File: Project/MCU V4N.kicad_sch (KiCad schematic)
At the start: 22 parts, among them J1 Conn_01x04, J10 Conn_01x01, J11 Conn_01x01, J2 Conn_01x01, J3 Conn_01x01, J4 Conn_01x01, J5 Conn_01x01, J6 Conn_01x01, J7 Conn_01x01, J8 Conn_01x01, J9 Conn_01x01, U53 STM32F072CBT6

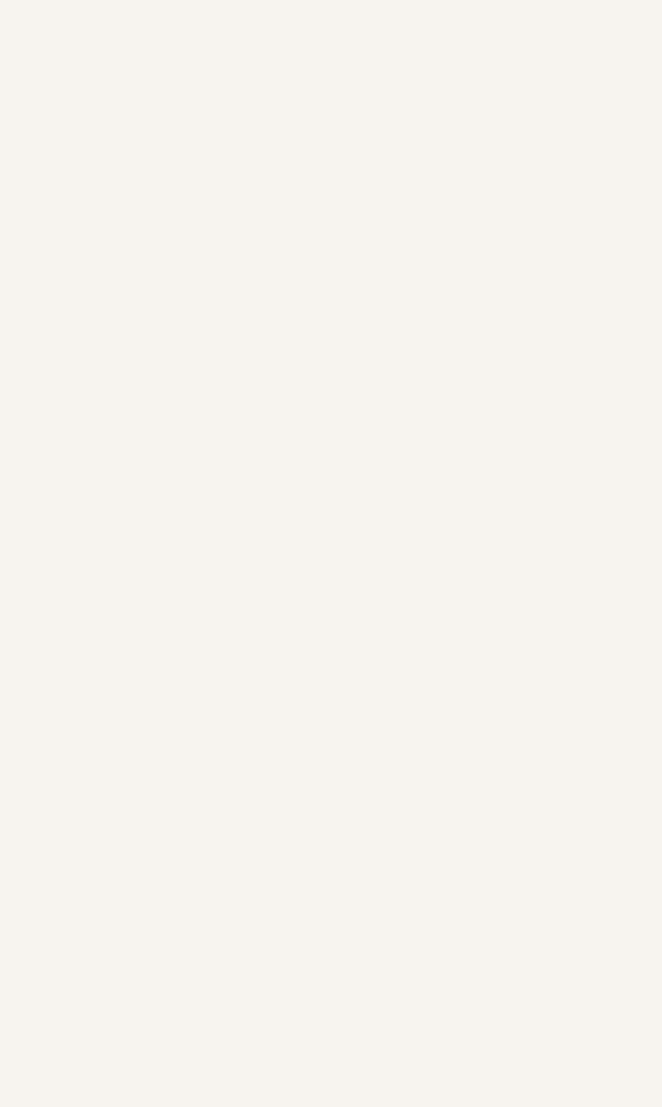
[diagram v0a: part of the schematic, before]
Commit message: revision work
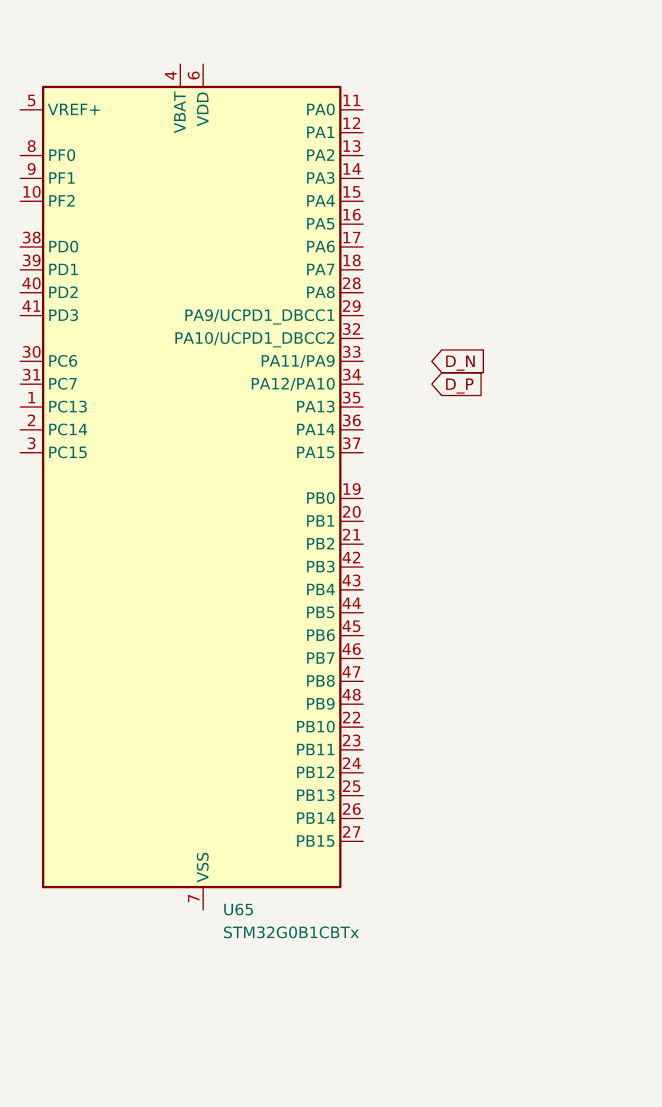
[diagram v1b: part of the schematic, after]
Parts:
- added U65: STM32G0B1CBTx, Package_QFP:LQFP-48_7x7mm_P0.5mm, symbol MCU_ST_STM32G0:STM32G0B1CBTx
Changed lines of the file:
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@@
+		)
+	)
+	(global_label "D_N"
+		(shape input)
+		(at -15.24 50.8 0)
+		(fields_autoplaced yes)
+		(effects
+			(font
+				(size 1.27 1.27)
+			)
+			(justify left)
+		)
+		(property "Intersheetrefs" "${INTERSHEET_REFS}"
+			(at -8.7661 50.8 0)
+			(effects
+				(font
+					(size 1.27 1.27)
+				)
+				(justify left)
+				(hide yes)
+			)
 		)
 	)
@@
 				)
 				(justify right)
+				(hide yes)
+			)
+		)
+	)
+	(global_label "D_P"
+		(shape input)
+		(at -15.24 53.34 0)
+		(fields_autoplaced yes)
+		(effects
+			(font
+				(size 1.27 1.27)
+			)
+			(justify left)
+		)
+		(property "Intersheetrefs" "${INTERSHEET_REFS}"
+			(at -8.8266 53.34 0)
+			(effects
+				(font
+					(size 1.27 1.27)
+				)
+				(justify left)
 				(hide yes)
 			)
@@
 					(unit 1)
 				)
+			)
+		)
+	)
+	(symbol
+		(lib_id "MCU_ST_STM32G0:STM32G0B1CBTx")
+		(at -43.18 66.04 0)
+		(unit 1)
+		(exclude_from_sim no)
+		(in_bom yes)
+		(on_board yes)
+		(dnp no)
+		(fields_autoplaced yes)
+		(property "Reference" "U65"
+			(at -38.4459 111.76 0)
+			(effects
+				(font
+					(size 1.27 1.27)
+				)
+				(justify left)
+			)
+		)
+		(property "Value" "STM32G0B1CBTx"
+			(at -38.4459 114.3 0)
+			(effects
+				(font
+					(size 1.27 1.27)
+				)
+				(justify left)
+			)
+		)
+		(property "Footprint" "Package_QFP:LQFP-48_7x7mm_P0.5mm"
+			(at -58.42 109.22 0)
+			(effects
+				(font
+					(size 1.27 1.27)
+				)
+				(justify right)
+				(hide yes)
+			)
+		)
+		(property "Datasheet" "https://www.st.com/resource/en/datasheet/stm32g0b1cb.pdf"
+			(at -43.18 66.04 0)
+			(effects
+				(font
+					(size 1.27 1.27)
+				)
+				(hide yes)
+			)
+		)
+		(property "Description" "STMicroelectronics Arm Cortex-M0+ MCU, 128KB flash, 144KB RAM, 64 MHz, 1.7-3.6V, 44 GPIO, LQFP48"
+			(at -43.18 66.04 0)
+			(effects
+				(font
+					(size 1.27 1.27)
+				)
+				(hide yes)
+			)
+		)
+		(pin "48"
+		)
+		(pin "28"
+		)
+		(pin "8"
+		)
+		(pin "31"
+		)
+		(pin "27"
+		)
+		(pin "29"
+		)
+		(pin "21"
+		)
+		(pin "24"
+		)
+		(pin "34"
+		)
+		(pin "11"
+		)
+		(pin "38"
+		)
+		(pin "37"
+		)
+		(pin "44"
+		)
+		(pin "30"
+		)
+		(pin "19"
+		)
+		(pin "22"
+		)
+		(pin "17"
+		)
+		(pin "1"
+		)
+		(pin "14"
+		)
+		(pin "32"
+		)
+		(pin "20"
+		)
+		(pin "10"
+		)
+		(pin "41"
+		)
+		(pin "47"
+		)
+		(pin "6"
+		)
+		(pin "46"
+		)
+		(pin "25"
+		)
+		(pin "45"
+		)
+		(pin "2"
+		)
+		(pin "3"
+		)
+		(pin "13"
+		)
+		(pin "43"
+		)
+		(pin "18"
+		)
+		(pin "35"
+		)
+		(pin "9"
+		)
+		(pin "33"
+		)
+		(pin "16"
+		)
+		(pin "7"
+		)
+		(pin "12"
+		)
+		(pin "15"
+		)
+		(pin "39"
+		)
+		(pin "42"
+		)
+		(pin "36"
+		)
+		(pin "5"
+		)
+		(pin "23"
+		)
+		(pin "26"
+		)
+		(pin "4"
+		)
+		(pin "40"
+		)
+		(instances
+			(project ""
+				(path "/7fa06d8b-464b-4050-a0fd-d319cc509390/00617548-7095-421c-9d05-30ad704b65f1"
+					(reference "U65")
+					(unit 1)
+				)

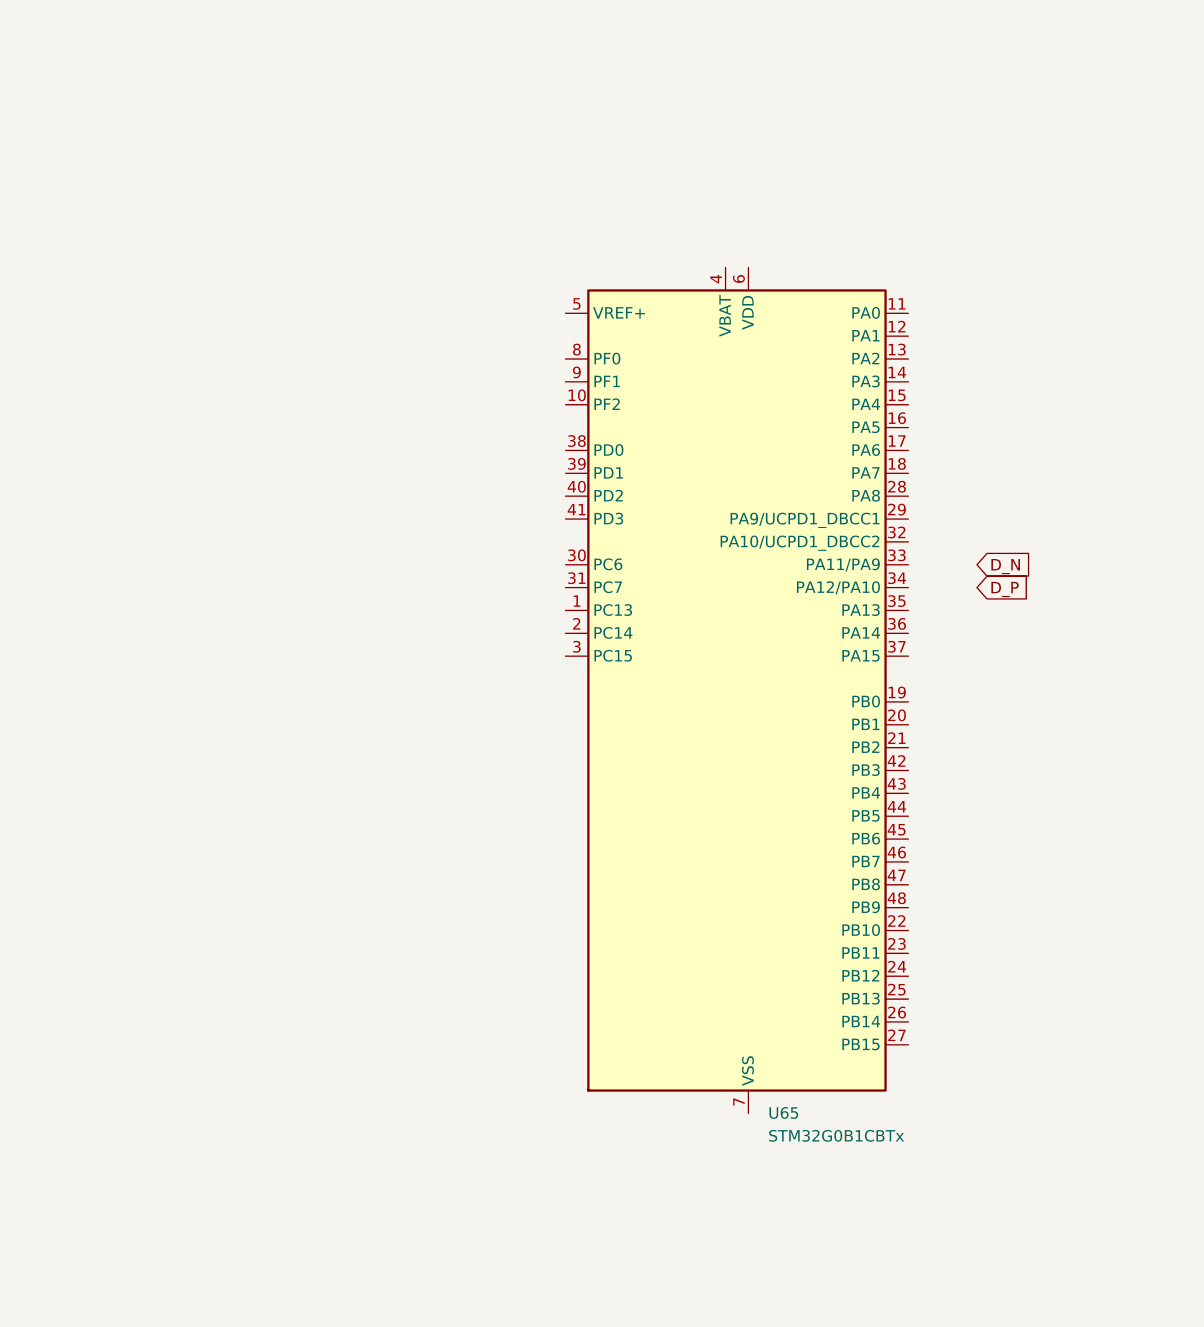
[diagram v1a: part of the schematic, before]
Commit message: wip
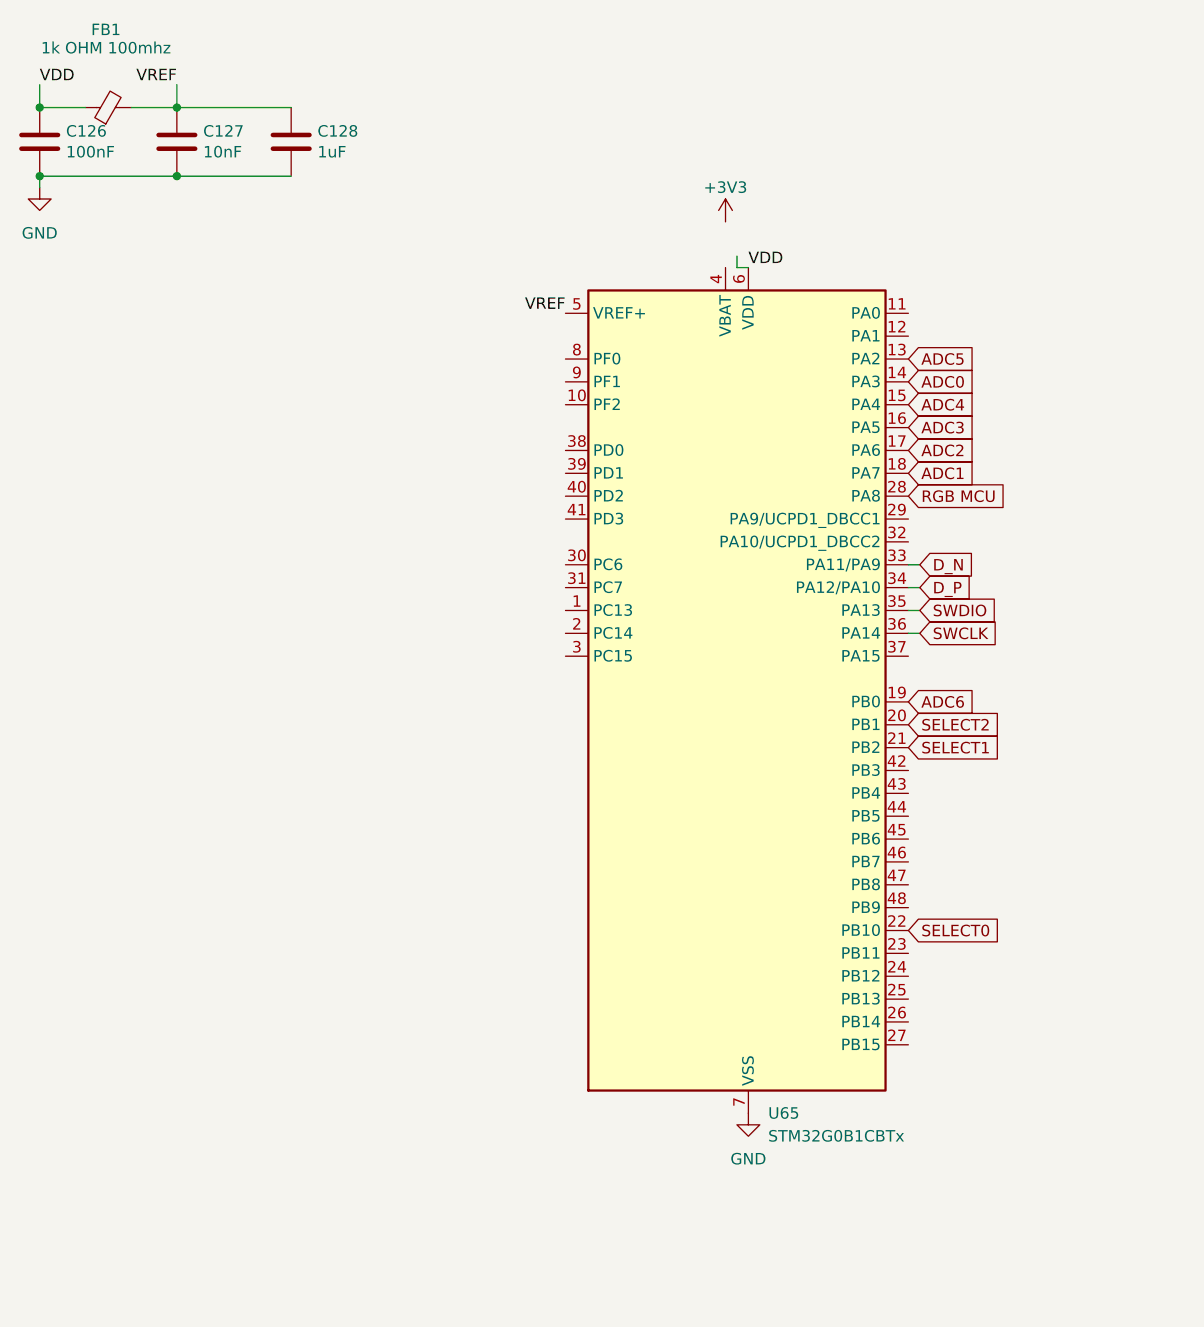
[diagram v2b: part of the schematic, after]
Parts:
- added C126: 100nF, Capacitor_SMD:C_0402_1005Metric, symbol Device:C
- added C127: 10nF, Capacitor_SMD:C_0402_1005Metric, symbol Device:C
- added C128: 1uF, Capacitor_SMD:C_0402_1005Metric, symbol Device:C
- added FB1: 1k OHM 100mhz, Fuse:Fuse_0402_1005Metric, symbol Device:FerriteBead_Small
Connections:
- net ADC0: now also U65.14 (PA3)
- net ADC1: now also U65.18 (PA7)
- net ADC2: now also U65.17 (PA6)
- net ADC3: now also U65.16 (PA5)
- net ADC4: now also U65.15 (PA4)
- net ADC5: now also U65.13 (PA2)
- net ADC6: now also U65.19 (PB0)
- net D_N: now also U65.33 (PA11/PA9)
- net D_P: now also U65.34 (PA12/PA10)
- net GND: now also U65.7 (VSS), C126.2, C127.2, C128.2
- net RGB MCU: now also U65.28 (PA8)
- net SELECT0: now also U65.22 (PB10)
- net SELECT1: now also U65.21 (PB2)
- net SELECT2: now also U65.20 (PB1)
- net SWCLK: now also U65.36 (PA14)
- net SWDIO: now also U65.35 (PA13)
- net VREF: now reaches U65.5 (VREF+)
- net VREF: now also C127.1, C128.1, FB1.2
- net VDD: now reaches U65.6 (VDD)
- net VDD: now also C126.1, FB1.1
